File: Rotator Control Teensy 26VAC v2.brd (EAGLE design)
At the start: 88.9 x 81.3 mm, 64 parts, among them K1 G5LE, K2 G5LE, K3 G5LE, Q1 BSS123, Q2 BSS123, Q3 BSS123, U1 SWITCH_TP_1825097-1, U2 MAX6959BAEE+, U3 SWITCH_TP_1825097-1, X1 Rotor, X2 26VAC

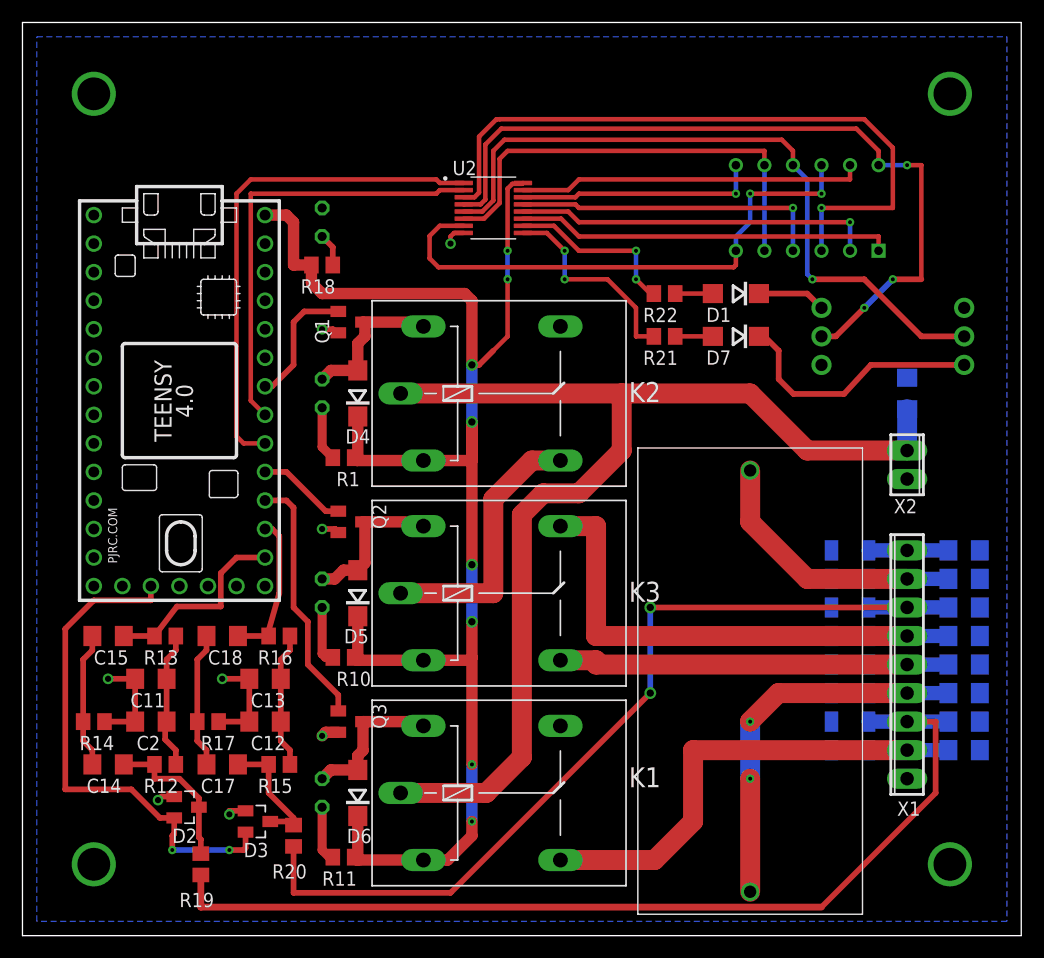
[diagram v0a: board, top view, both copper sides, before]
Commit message: Released this version to OshPark for fab
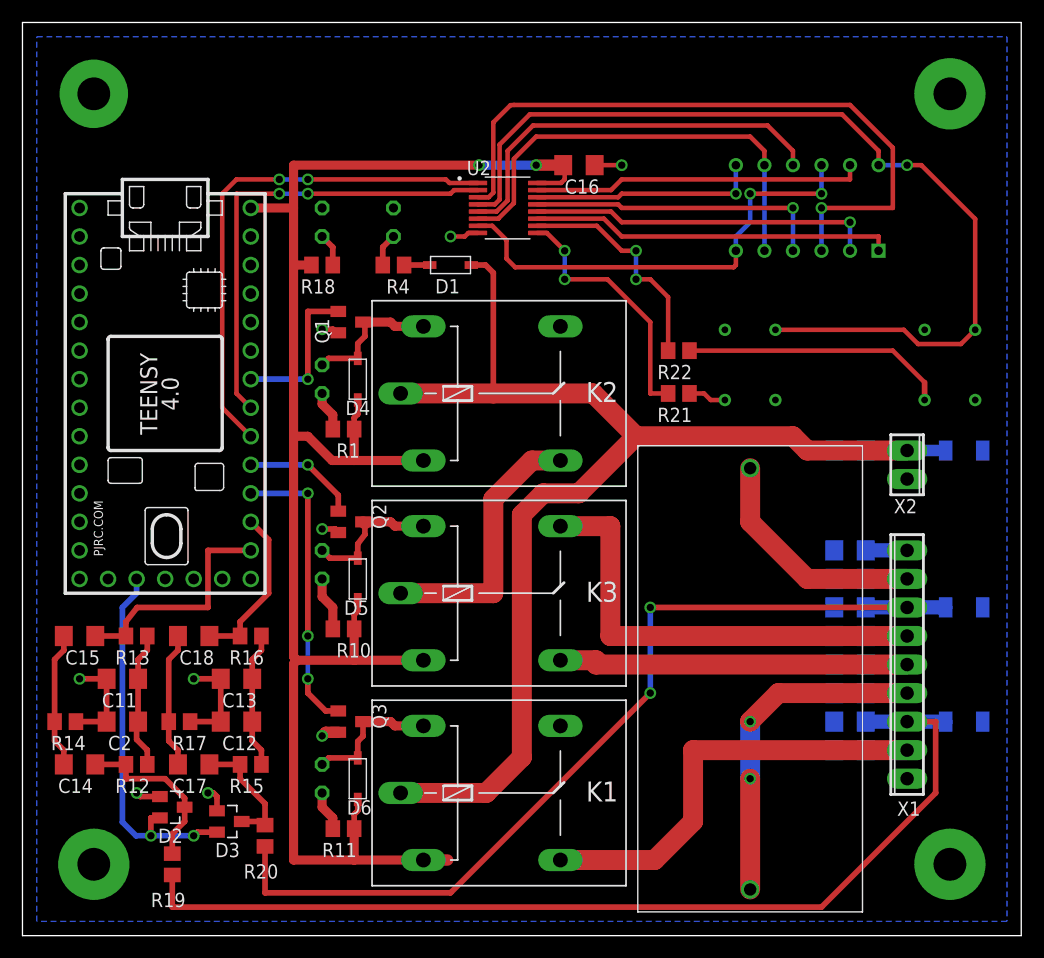
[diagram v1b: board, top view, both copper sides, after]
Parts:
- removed D7: 1N4148, diode:DO214AC
- removed R5, R6, R8, R9: VARISTORCN1206, varistor:CT/CN1206
- removed U1, U3: SWITCH_TP_1825097-1, my-library:SW3-TOGGLE-2POL_P100
- added C16: .1, rcl:C1206
- added LED4: 26VAC, led:LED3MM
- added U$2, U$3: SWITCH_AEXIT_6X6X9.5, my-library:PUSHBUTTON_6X6
- D1, D4, D5, D6: device diode:DO214AC -> adafruit:SOD-123
- R4: value VARISTORCN1206 -> 3600; device varistor:CT/CN1206 -> rcl:R0805
- moved R4 55.7 mm to (33.0, 59.7), flipped to the top
- moved R2 28.5 mm to (83.8, 43.2), turned to 180 degrees
- moved D1 25.5 mm to (38.1, 59.7), turned to 0 degrees
- moved C1 10.2 mm to (73.7, 16.5), turned to 0 degrees
- moved C3 10.2 mm to (73.7, 24.1), turned to 0 degrees
- moved C4 10.2 mm to (73.7, 26.7), turned to 0 degrees
- moved C5 10.2 mm to (73.7, 34.3), turned to 0 degrees
- moved C6 10.2 mm to (73.7, 29.2), turned to 0 degrees
- moved C7 10.2 mm to (73.7, 19.1), turned to 0 degrees
- moved C8 10.2 mm to (73.7, 21.6), turned to 0 degrees
- moved C9 10.2 mm to (73.7, 31.8), turned to 0 degrees
- moved R3 10.2 mm to (83.8, 19.1), turned to 180 degrees
- moved R7 10.2 mm to (83.8, 29.2), turned to 180 degrees
- moved C10 7.18 mm to (73.7, 43.2), turned to 0 degrees
- moved R21 5.24 mm to (58.4, 48.3)
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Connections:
- net +5V: now also C16.1
- net 26VAC: now also D1.A, R2.1
- net BRAKE: no longer R2.1
- net CAP1: no longer R4.1
- net CAP2: no longer R8.1
- net DIG0: now also U$2.P$1, U$3.P$1; no longer U1.2
- net DIG1: no longer U3.2
- net GND: now also C16.2, LED4.K; no longer R4.2, R5.2, R6.2, R8.2, R9.2
- net LEFT: no longer R6.1
- net N$19: now also U$3.P$2; no longer D7.A
- net N$20: now also U$2.P$2; no longer D1.A
- net N$24: now also R4.2; no longer U1.3
- net N$25: now also LED4.A, R4.1; no longer D7.C, U3.3
- net N/C: no longer R9.1
- net RIGHT: no longer R5.1
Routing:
- net DIG1: track 62.7 -> 36.0 mm, vias 1 -> 0
- net N$20: track 3.35 -> 23.7 mm
- net N$25: track 23.0 -> 2.93 mm
- net DIG0: track 69.6 -> 83.7 mm, vias 3 -> 1
- net 26VAC: track 100.9 -> 114.0 mm
- net +3V3: track 45.9 -> 33.6 mm
- net +5V: track 139.3 -> 149.4 mm, vias 8 -> 2
- net DIG3: track 48.8 -> 41.3 mm
- net N$16: track 15.6 -> 20.5 mm
- net N$15: track 18.4 -> 22.8 mm
- net GND: track 28.4 -> 32.5 mm, vias 12 -> 13
- net N$24: track 6.10 -> 2.28 mm
- net N$12: track 22.6 -> 26.2 mm, vias 0 -> 3
- net CAP1: track 37.3 -> 33.7 mm
- net RIGHT: track 38.4 -> 34.9 mm
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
